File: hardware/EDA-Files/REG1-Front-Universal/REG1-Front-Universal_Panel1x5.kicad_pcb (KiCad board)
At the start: 2 copper layers, 106.3 x 52.8 mm, 60 parts, among them J1 Conn_02x04_Odd_Even, SW1 Prog, SW2 Func, SW3 Res, SW4 BL

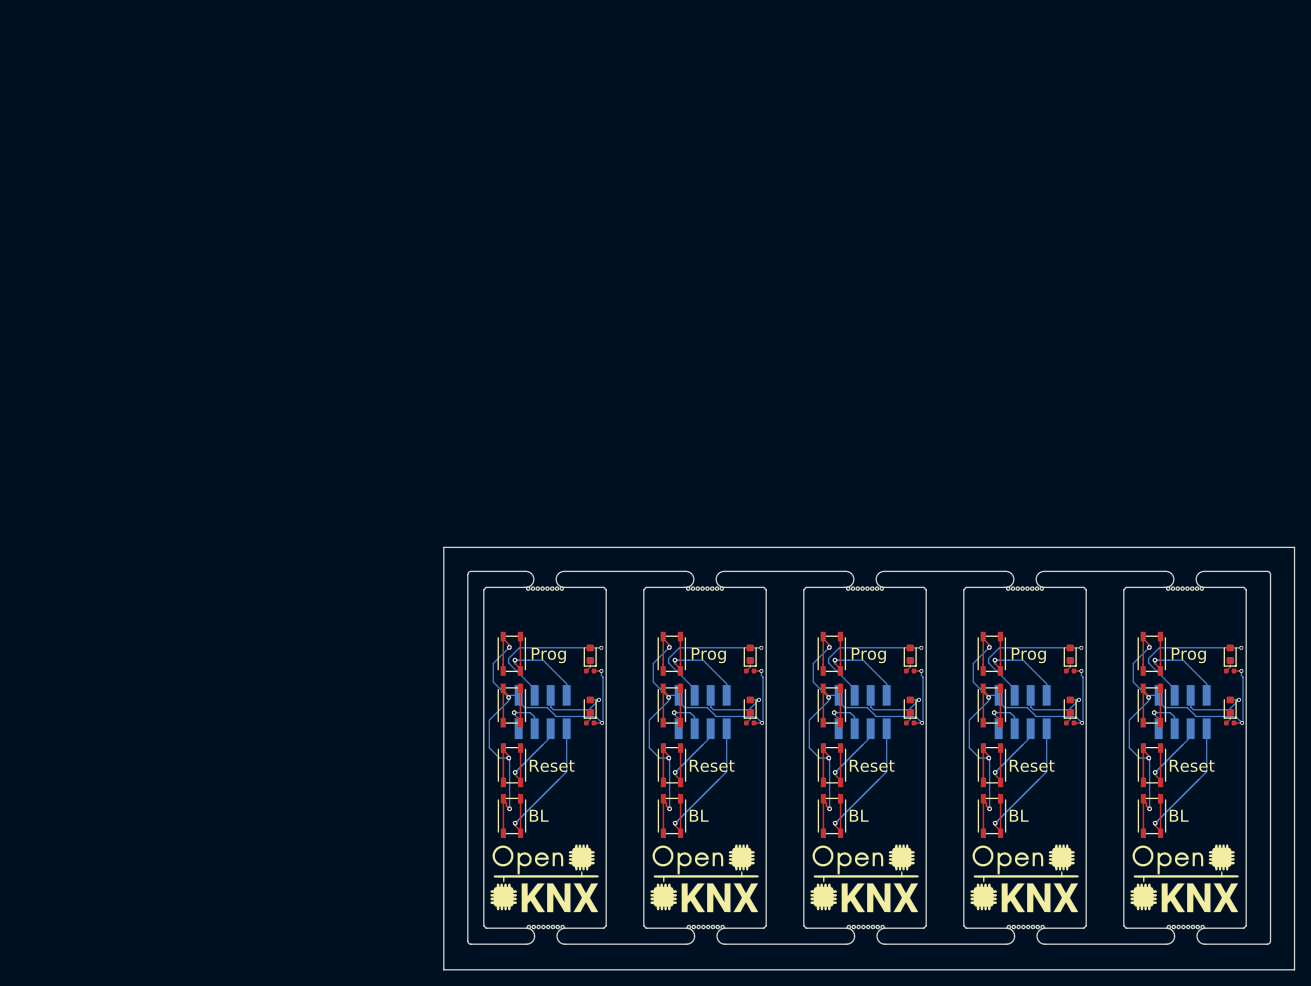
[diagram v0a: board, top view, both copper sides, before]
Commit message: REG1-Front-Universal V01.00
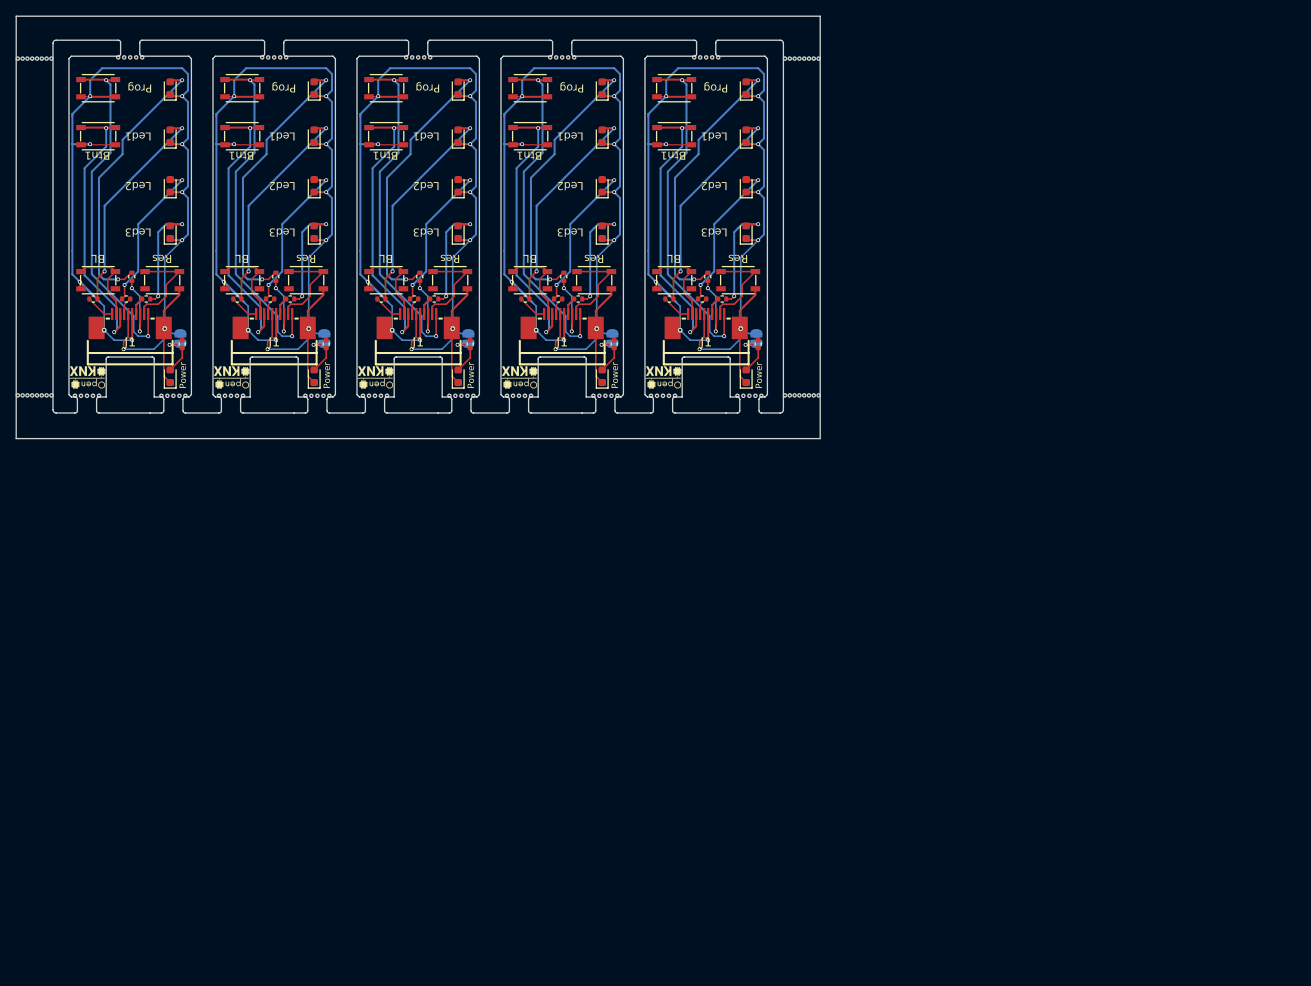
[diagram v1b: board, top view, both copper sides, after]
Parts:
- removed the D1 at (191.5, 117.8)
- removed the D1 at (171.5, 117.8)
- removed the D1 at (151.5, 117.8)
- removed the D1 at (131.5, 117.8)
- removed the D2 at (191.5, 124.2)
- removed the D2 at (171.5, 124.2)
- removed the D2 at (151.5, 124.2)
- removed the D2 at (131.5, 124.2)
- removed the G*** at (185.8, 146.4)
- removed the G*** at (165.8, 146.4)
- removed the G*** at (145.8, 146.4)
- removed the G*** at (125.8, 146.4)
- removed the G*** at (105.8, 146.4)
- removed the J1 at (185.6, 125.0)
- removed the J1 at (165.6, 125.0)
- removed the J1 at (145.6, 125.0)
- removed the J1 at (125.6, 125.0)
- removed the J1 at (105.6, 125.0)
- removed the R1 at (191.5, 119.8)
- removed the R1 at (171.5, 119.8)
- removed the R1 at (151.5, 119.8)
- removed the R1 at (131.5, 119.8)
- removed the R2 at (191.5, 126.3)
- removed the R2 at (171.5, 126.3)
- removed the R2 at (151.5, 126.3)
- removed the R2 at (131.5, 126.3)
- removed the SW1 at (181.7, 117.7)
- removed the SW1 at (161.7, 117.7)
- removed the SW1 at (141.7, 117.7)
- removed the SW1 at (121.7, 117.7)
- removed the SW2 at (181.7, 124.2)
- removed the SW2 at (161.7, 124.2)
- removed the SW2 at (141.7, 124.2)
- removed the SW2 at (121.7, 124.2)
- removed the SW3 at (181.7, 131.6)
- removed the SW3 at (161.7, 131.6)
- removed the SW3 at (141.7, 131.6)
- removed the SW3 at (121.7, 131.6)
- removed the SW4 at (181.7, 138.0)
- removed the SW4 at (161.7, 138.0)
- removed the SW4 at (141.7, 138.0)
- removed the SW4 at (121.7, 138.0)
- removed the mouse-bite at (186.4, 151.8)
- removed the mouse-bite at (105.3, 109.5)
- removed the mouse-bite at (166.4, 151.8)
- removed the mouse-bite at (146.4, 151.8)
- removed the mouse-bite at (126.5, 151.8)
- removed the mouse-bite at (185.3, 109.5)
- removed the mouse-bite at (165.3, 109.5)
- removed the mouse-bite at (145.3, 109.5)
- removed the mouse-bite at (125.3, 109.5)
- removed the mouse-bite at (106.5, 151.8)
- added D1: Prog, LED_SMD:LED_0603_1608Metric, F.Cu at (131.0, 47.0)
- added D1: Prog, LED_SMD:LED_0603_1608Metric, F.Cu at (77.0, 47.0)
- added D1: Prog, LED_SMD:LED_0603_1608Metric, F.Cu at (113.0, 47.0)
- added D1: Prog, LED_SMD:LED_0603_1608Metric, F.Cu at (95.0, 47.0)
- added D2: Led1, LED_SMD:LED_0603_1608Metric, F.Cu at (131.0, 53.0)
- added D2: Led1, LED_SMD:LED_0603_1608Metric, F.Cu at (95.0, 53.0)
- added D2: Led1, LED_SMD:LED_0603_1608Metric, F.Cu at (113.0, 53.0)
- added D2: Led1, LED_SMD:LED_0603_1608Metric, F.Cu at (77.0, 53.0)
- added D3: Led2, LED_SMD:LED_0603_1608Metric, F.Cu at (59.0, 59.2)
- added D3: Led2, LED_SMD:LED_0603_1608Metric, F.Cu at (95.0, 59.2)
- added D3: Led2, LED_SMD:LED_0603_1608Metric, F.Cu at (77.0, 59.2)
- added D3: Led2, LED_SMD:LED_0603_1608Metric, F.Cu at (113.0, 59.2)
- added D3: Led2, LED_SMD:LED_0603_1608Metric, F.Cu at (131.0, 59.2)
- added D4: Led3, LED_SMD:LED_0603_1608Metric, F.Cu at (131.0, 65.0)
- added D4: Led3, LED_SMD:LED_0603_1608Metric, F.Cu at (113.0, 65.0)
- added D4: Led3, LED_SMD:LED_0603_1608Metric, F.Cu at (95.0, 65.0)
- added D4: Led3, LED_SMD:LED_0603_1608Metric, F.Cu at (77.0, 65.0)
- added D4: Led3, LED_SMD:LED_0603_1608Metric, F.Cu at (59.0, 65.0)
- added D5: Power, LED_SMD:LED_0603_1608Metric, F.Cu at (113.0, 83.0)
- added D5: Power, LED_SMD:LED_0603_1608Metric, F.Cu at (59.0, 83.0)
- added D5: Power, LED_SMD:LED_0603_1608Metric, F.Cu at (95.0, 83.0)
- added D5: Power, LED_SMD:LED_0603_1608Metric, F.Cu at (77.0, 83.0)
- added D5: Power, LED_SMD:LED_0603_1608Metric, F.Cu at (131.0, 83.0)
- added G***: LOGO, OpenKNX:OpenKNX_Logo_05x03, F.Cu at (120.7, 83.0)
- added G***: LOGO, OpenKNX:OpenKNX_Logo_07x05, B.Cu at (106.0, 50.6)
- added G***: LOGO, OpenKNX:OpenKNX_Logo_05x03, F.Cu at (66.7, 83.0)
- added G***: LOGO, OpenKNX:OpenKNX_Logo_05x03, F.Cu at (102.7, 83.0)
- added G***: LOGO, OpenKNX:OpenKNX_Logo_05x03, F.Cu at (84.7, 83.0)
- added G***: LOGO, OpenKNX:OpenKNX_Logo_05x03, F.Cu at (48.7, 83.0)
- added G***: LOGO, OpenKNX:OpenKNX_Logo_07x05, B.Cu at (70.0, 50.6)
- added G***: LOGO, OpenKNX:OpenKNX_Logo_07x05, B.Cu at (88.0, 50.6)
- added G***: LOGO, OpenKNX:OpenKNX_Logo_07x05, B.Cu at (52.0, 50.6)
- added G***: LOGO, OpenKNX:OpenKNX_Logo_07x05, B.Cu at (124.0, 50.6)
- added J1: Frontpanel, EasyEDAModLib:C11050_FPC-SMD_P0.5-10P_LSXJ-H2.0-10P, F.Cu at (72.0, 76.1)
- added J1: Frontpanel, EasyEDAModLib:C11050_FPC-SMD_P0.5-10P_LSXJ-H2.0-10P, F.Cu at (54.0, 76.1)
- added J1: Frontpanel, EasyEDAModLib:C11050_FPC-SMD_P0.5-10P_LSXJ-H2.0-10P, F.Cu at (90.0, 76.1)
- added J1: Frontpanel, EasyEDAModLib:C11050_FPC-SMD_P0.5-10P_LSXJ-H2.0-10P, F.Cu at (108.0, 76.1)
- added J1: Frontpanel, EasyEDAModLib:C11050_FPC-SMD_P0.5-10P_LSXJ-H2.0-10P, F.Cu at (126.0, 76.1)
- added JP1: PowerLED Jumper, Jumper:SolderJumper-2_P1.3mm_Open_RoundedPad1.0x1.5mm, B.Cu at (60.3, 78.3)
- added JP1: PowerLED Jumper, Jumper:SolderJumper-2_P1.3mm_Open_RoundedPad1.0x1.5mm, B.Cu at (114.3, 78.3)
- added JP1: PowerLED Jumper, Jumper:SolderJumper-2_P1.3mm_Open_RoundedPad1.0x1.5mm, B.Cu at (96.3, 78.3)
- added JP1: PowerLED Jumper, Jumper:SolderJumper-2_P1.3mm_Open_RoundedPad1.0x1.5mm, B.Cu at (132.3, 78.3)
- added JP1: PowerLED Jumper, Jumper:SolderJumper-2_P1.3mm_Open_RoundedPad1.0x1.5mm, B.Cu at (78.3, 78.3)
- added R1: 2k2, Resistor_SMD:R_0402_1005Metric, F.Cu at (126.2, 70.6)
- added R1: 2k2, Resistor_SMD:R_0402_1005Metric, F.Cu at (72.2, 70.6)
- added R1: 2k2, Resistor_SMD:R_0402_1005Metric, F.Cu at (108.2, 70.6)
- added R1: 2k2, Resistor_SMD:R_0402_1005Metric, F.Cu at (90.2, 70.6)
- added R2: 2k2, Resistor_SMD:R_0402_1005Metric, F.Cu at (121.4, 73.3)
- added R2: 2k2, Resistor_SMD:R_0402_1005Metric, F.Cu at (85.4, 73.3)
- added R2: 2k2, Resistor_SMD:R_0402_1005Metric, F.Cu at (103.4, 73.3)
- added R2: 2k2, Resistor_SMD:R_0402_1005Metric, F.Cu at (67.4, 73.3)
- added R3: 2k2, Resistor_SMD:R_0402_1005Metric, F.Cu at (89.5, 73.3)
- added R3: 2k2, Resistor_SMD:R_0402_1005Metric, F.Cu at (107.5, 73.3)
- added R3: 2k2, Resistor_SMD:R_0402_1005Metric, F.Cu at (71.5, 73.3)
- added R3: 2k2, Resistor_SMD:R_0402_1005Metric, F.Cu at (53.5, 73.3)
- added R3: 2k2, Resistor_SMD:R_0402_1005Metric, F.Cu at (125.5, 73.3)
- added R4: 2k2, Resistor_SMD:R_0402_1005Metric, F.Cu at (56.0, 73.3)
- added R4: 2k2, Resistor_SMD:R_0402_1005Metric, F.Cu at (110.0, 73.3)
- added R4: 2k2, Resistor_SMD:R_0402_1005Metric, F.Cu at (92.0, 73.3)
- added R4: 2k2, Resistor_SMD:R_0402_1005Metric, F.Cu at (74.0, 73.3)
- added R4: 2k2, Resistor_SMD:R_0402_1005Metric, F.Cu at (128.0, 73.3)
- added R5: 2k2, Resistor_SMD:R_0402_1005Metric, F.Cu at (132.5, 79.0)
- added R5: 2k2, Resistor_SMD:R_0402_1005Metric, F.Cu at (114.5, 79.0)
- added R5: 2k2, Resistor_SMD:R_0402_1005Metric, F.Cu at (96.5, 79.0)
- added R5: 2k2, Resistor_SMD:R_0402_1005Metric, F.Cu at (60.5, 79.0)
- added R5: 2k2, Resistor_SMD:R_0402_1005Metric, F.Cu at (78.5, 79.0)
- added SW1: Prog, EasyEDAModLib:C455282_SW-SMD_4P-L4.2-W3.3-P2.15-LS5.1, F.Cu at (104.0, 47.0)
- added SW1: Prog, EasyEDAModLib:C455282_SW-SMD_4P-L4.2-W3.3-P2.15-LS5.1, F.Cu at (122.0, 47.0)
- added SW1: Prog, EasyEDAModLib:C455282_SW-SMD_4P-L4.2-W3.3-P2.15-LS5.1, F.Cu at (86.0, 47.0)
- added SW1: Prog, EasyEDAModLib:C455282_SW-SMD_4P-L4.2-W3.3-P2.15-LS5.1, F.Cu at (68.0, 47.0)
- added SW2: Btn1, EasyEDAModLib:C455282_SW-SMD_4P-L4.2-W3.3-P2.15-LS5.1, F.Cu at (86.0, 53.0)
- added SW2: Btn1, EasyEDAModLib:C455282_SW-SMD_4P-L4.2-W3.3-P2.15-LS5.1, F.Cu at (104.0, 53.0)
- added SW2: Btn1, EasyEDAModLib:C455282_SW-SMD_4P-L4.2-W3.3-P2.15-LS5.1, F.Cu at (122.0, 53.0)
- added SW2: Btn1, EasyEDAModLib:C455282_SW-SMD_4P-L4.2-W3.3-P2.15-LS5.1, F.Cu at (68.0, 53.0)
- added SW3: Res, EasyEDAModLib:C455282_SW-SMD_4P-L4.2-W3.3-P2.15-LS5.1, F.Cu at (76.0, 71.0)
- added SW3: Res, EasyEDAModLib:C455282_SW-SMD_4P-L4.2-W3.3-P2.15-LS5.1, F.Cu at (94.0, 71.0)
- added SW3: Res, EasyEDAModLib:C455282_SW-SMD_4P-L4.2-W3.3-P2.15-LS5.1, F.Cu at (130.0, 71.0)
- added SW3: Res, EasyEDAModLib:C455282_SW-SMD_4P-L4.2-W3.3-P2.15-LS5.1, F.Cu at (112.0, 71.0)
- added SW4: BL, EasyEDAModLib:C455282_SW-SMD_4P-L4.2-W3.3-P2.15-LS5.1, F.Cu at (68.0, 71.0)
- added SW4: BL, EasyEDAModLib:C455282_SW-SMD_4P-L4.2-W3.3-P2.15-LS5.1, F.Cu at (122.0, 71.0)
- added SW4: BL, EasyEDAModLib:C455282_SW-SMD_4P-L4.2-W3.3-P2.15-LS5.1, F.Cu at (104.0, 71.0)
- added SW4: BL, EasyEDAModLib:C455282_SW-SMD_4P-L4.2-W3.3-P2.15-LS5.1, F.Cu at (86.0, 71.0)
- added e: VAL**, DomsKiCADLib:mouse-bite-5.00mm-frame, F.Cu at (41.5, 43.3)
- added e: VAL**, DomsKiCADLib:mouse-bite-5.00mm-frame, F.Cu at (137.4, 43.3)
- added mouse-bite: mouse-bite-2.00mm-slot_1side, DomsKiCADLib:mouse-bite-2.00mm-slot_1side, F.Cu at (48.6, 86.2)
- added mouse-bite: mouse-bite-2.00mm-slot_1side, DomsKiCADLib:mouse-bite-2.00mm-slot_1side, F.Cu at (131.4, 86.2)
- added mouse-bite: VAL**, DomsKiCADLib:mouse-bite-5.00mm-frame, F.Cu at (137.4, 85.4)
- added mouse-bite: mouse-bite-2.00mm-slot_1side, DomsKiCADLib:mouse-bite-2.00mm-slot_1side, F.Cu at (54.0, 42.4)
- added mouse-bite: mouse-bite-2.00mm-slot_1side, DomsKiCADLib:mouse-bite-2.00mm-slot_1side, F.Cu at (95.4, 86.2)
- added mouse-bite: mouse-bite-2.00mm-slot_1side, DomsKiCADLib:mouse-bite-2.00mm-slot_1side, F.Cu at (72.0, 42.4)
- added mouse-bite: mouse-bite-2.00mm-slot_1side, DomsKiCADLib:mouse-bite-2.00mm-slot_1side, F.Cu at (66.6, 86.2)
- added mouse-bite: mouse-bite-2.00mm-slot_1side, DomsKiCADLib:mouse-bite-2.00mm-slot_1side, F.Cu at (126.0, 42.4)
- added mouse-bite: mouse-bite-2.00mm-slot_1side, DomsKiCADLib:mouse-bite-2.00mm-slot_1side, F.Cu at (84.6, 86.2)
- added mouse-bite: mouse-bite-2.00mm-slot_1side, DomsKiCADLib:mouse-bite-2.00mm-slot_1side, F.Cu at (77.4, 86.2)
- added mouse-bite: VAL**, DomsKiCADLib:mouse-bite-5.00mm-frame, F.Cu at (41.5, 85.4)
- added mouse-bite: mouse-bite-2.00mm-slot_1side, DomsKiCADLib:mouse-bite-2.00mm-slot_1side, F.Cu at (120.6, 86.2)
- added mouse-bite: mouse-bite-2.00mm-slot_1side, DomsKiCADLib:mouse-bite-2.00mm-slot_1side, F.Cu at (113.4, 86.2)
- added mouse-bite: mouse-bite-2.00mm-slot_1side, DomsKiCADLib:mouse-bite-2.00mm-slot_1side, F.Cu at (108.0, 42.4)
- added mouse-bite: mouse-bite-2.00mm-slot_1side, DomsKiCADLib:mouse-bite-2.00mm-slot_1side, F.Cu at (59.4, 86.2)
- added mouse-bite: mouse-bite-2.00mm-slot_1side, DomsKiCADLib:mouse-bite-2.00mm-slot_1side, F.Cu at (102.6, 86.2)
- added mouse-bite: mouse-bite-2.00mm-slot_1side, DomsKiCADLib:mouse-bite-2.00mm-slot_1side, F.Cu at (90.0, 42.4)
- D2: value Func -> Led1
- R1, R2: value R -> 2k2
- SW1, SW3, SW4: footprint sirsydom:SW_Push_Xunpu_TS-1089S -> EasyEDAModLib:C455282_SW-SMD_4P-L4.2-W3.3-P2.15-LS5.1
- SW2: value Func -> Btn1; footprint sirsydom:SW_Push_Xunpu_TS-1089S -> EasyEDAModLib:C455282_SW-SMD_4P-L4.2-W3.3-P2.15-LS5.1
- moved D2 88.5 mm to (59.0, 53.0)
- moved D1 88.1 mm to (59.0, 47.0)
- moved SW2 88.0 mm to (50.0, 53.0), turned to 0 degrees
- moved SW1 87.6 mm to (50.0, 47.0), turned to 0 degrees
- moved SW4 84.6 mm to (50.0, 71.0), turned to 0 degrees
- moved R2 81.6 mm to (49.4, 73.3)
- moved R1 75.6 mm to (54.2, 70.6), turned to -90 degrees
- moved SW3 74.7 mm to (58.0, 71.0), turned to 0 degrees
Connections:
- D1 pad 1: Net-(D1-Pad1) -> GND
- D1 pad 2: PROGLED -> Net-(D1-A)
- D2 pad 1: Net-(D2-Pad1) -> GND
- D2 pad 2: GPIO03 -> Net-(D2-A)
- R1 pad 1: GND -> Net-(D1-A)
- R1 pad 2: Net-(D1-Pad1) -> GPIO25
- R2 pad 1: GND -> Net-(D2-A)
- R2 pad 2: Net-(D2-Pad1) -> GPIO6
- SW1 pad 1: PROGBTN -> GPIO23
- SW2 pad 1: GPIO24 -> GPIO7
- SW4 pad 1: BOOTSEL_F -> BOOTSEL
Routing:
- net GND: track 352.6 -> 606.9 mm, vias 30 -> 50
- net GPIO23: track 0.00 -> 219.8 mm, vias 0 -> 10
- net GPIO7: track 0.00 -> 176.6 mm, vias 0 -> 10
- net Net-(D1-A): track 0.00 -> 174.6 mm, vias 0 -> 10
- net BOOTSEL_F: track 140.1 -> 0.00 mm, vias 5 -> 0
- net Net-(D2-A): track 0.00 -> 137.0 mm, vias 0 -> 10
- net PROGLED: track 97.5 -> 0.00 mm, vias 5 -> 0
- net Net-(D3-A): track 0.00 -> 97.5 mm, vias 0 -> 10
- net PROGBTN: track 75.4 -> 0.00 mm, vias 5 -> 0
- net Net-(D4-A): track 0.00 -> 70.7 mm, vias 0 -> 10
- net +3.3V: track 0.00 -> 62.7 mm, vias 0 -> 5
- net BOOTSEL: track 0.00 -> 54.4 mm
- net GPIO03: track 46.3 -> 0.00 mm, vias 5 -> 0
- net GPIO25: track 0.00 -> 46.1 mm, vias 0 -> 10
- net GPIO24: track 50.5 -> 11.0 mm, vias 5 -> 0
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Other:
- board size 106.3 x 52.8 mm -> 100.5 x 52.8 mm
- net class Default removed
- rule pad_to_mask_clearance: 0.051 -> 0.038
- board text added: "REG1-Front-Universal V01.00 (c) Ing-Dom, 2023"
- board text removed: "3V3"
- board text removed: "BL"
- board text removed: "GND"
- board text removed: "GP24"
- board text removed: "GP3"
- board text removed: "PBTN"
- board text removed: "PLED"
- board text removed: "Prog"
- board text removed: "REG1-Front-Universal V00.02 © Ing-Dom, 2022"
- board text removed: "RES"
- board text removed: "Reset"

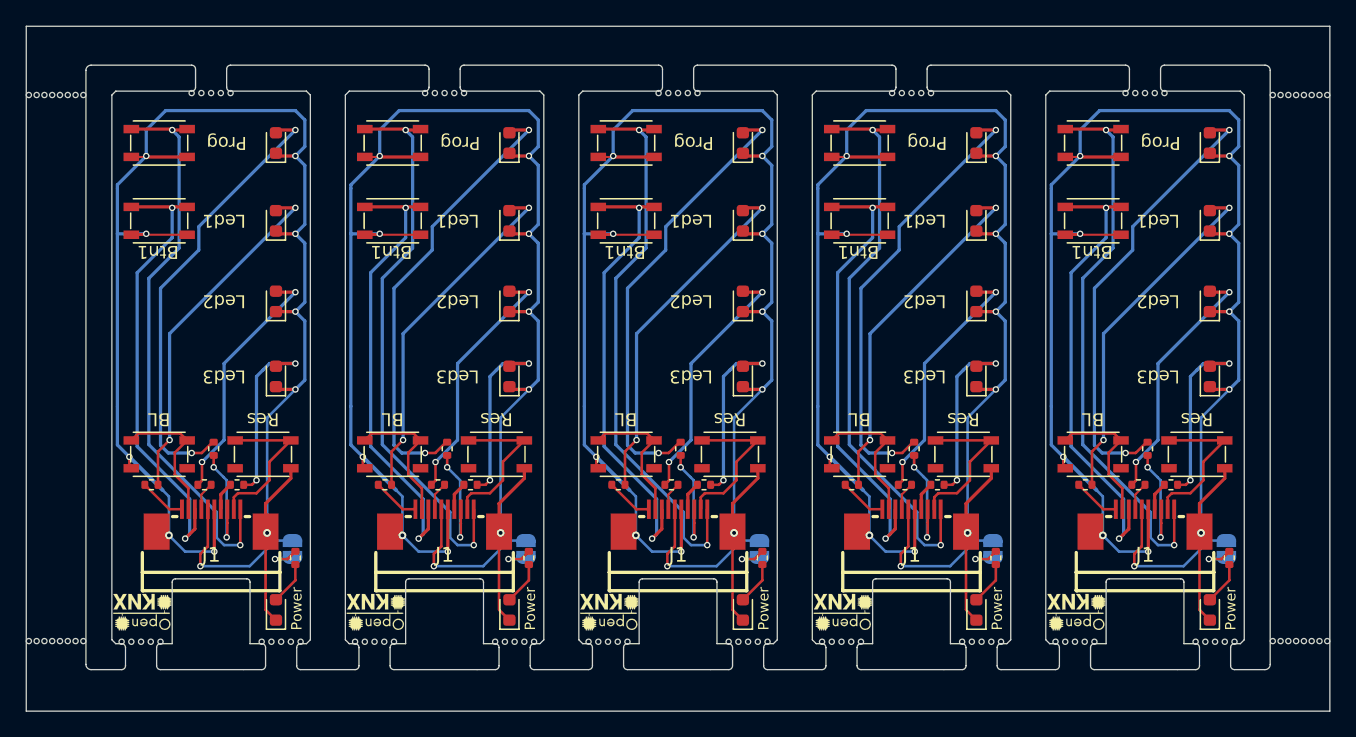
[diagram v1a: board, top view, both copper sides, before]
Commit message: new V01.00 (some 0.1 bigger)
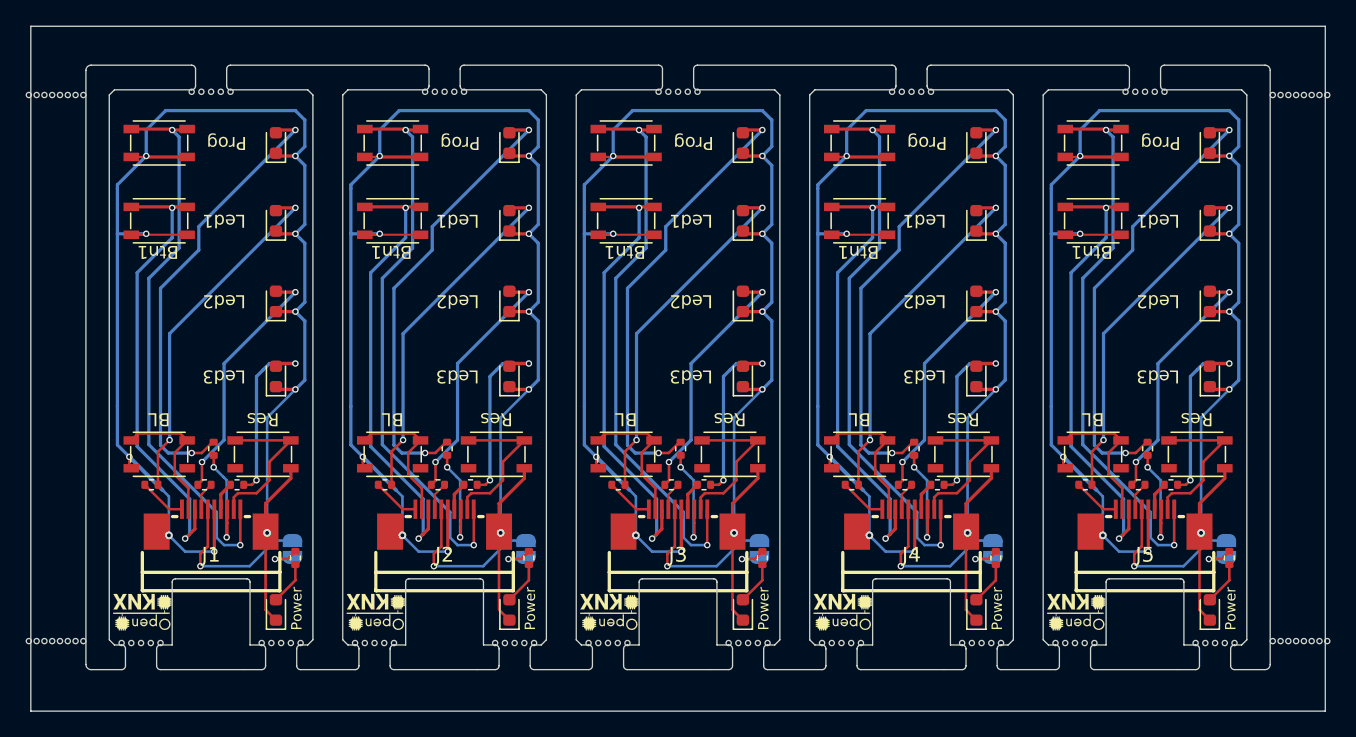
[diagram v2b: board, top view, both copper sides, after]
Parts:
- removed the D1 at (131.0, 47.0)
- removed the D1 at (77.0, 47.0)
- removed the D1 at (113.0, 47.0)
- removed the D1 at (95.0, 47.0)
- removed the D2 at (131.0, 53.0)
- removed the D2 at (95.0, 53.0)
- removed the D2 at (113.0, 53.0)
- removed the D2 at (77.0, 53.0)
- removed the D3 at (95.0, 59.2)
- removed the D3 at (77.0, 59.2)
- removed the D3 at (113.0, 59.2)
- removed the D3 at (131.0, 59.2)
- removed the D4 at (131.0, 65.0)
- removed the D4 at (113.0, 65.0)
- removed the D4 at (95.0, 65.0)
- removed the D4 at (77.0, 65.0)
- removed the D5 at (113.0, 83.0)
- removed the D5 at (95.0, 83.0)
- removed the D5 at (77.0, 83.0)
- removed the D5 at (131.0, 83.0)
- removed the G*** at (120.7, 83.0)
- removed the G*** at (106.0, 50.6)
- removed the G*** at (66.7, 83.0)
- removed the G*** at (102.7, 83.0)
- removed the G*** at (84.7, 83.0)
- removed the G*** at (70.0, 50.6)
- removed the G*** at (88.0, 50.6)
- removed the G*** at (124.0, 50.6)
- removed the J1 at (72.0, 76.1)
- removed the J1 at (90.0, 76.1)
- removed the J1 at (108.0, 76.1)
- removed the J1 at (126.0, 76.1)
- removed the JP1 at (114.3, 78.3)
- removed the JP1 at (96.3, 78.3)
- removed the JP1 at (132.3, 78.3)
- removed the JP1 at (78.3, 78.3)
- removed the R1 at (126.2, 70.6)
- removed the R1 at (72.2, 70.6)
- removed the R1 at (108.2, 70.6)
- removed the R1 at (90.2, 70.6)
- removed the R2 at (121.4, 73.3)
- removed the R2 at (85.4, 73.3)
- removed the R2 at (103.4, 73.3)
- removed the R2 at (67.4, 73.3)
- removed the R3 at (89.5, 73.3)
- removed the R3 at (107.5, 73.3)
- removed the R3 at (71.5, 73.3)
- removed the R3 at (125.5, 73.3)
- removed the R4 at (110.0, 73.3)
- removed the R4 at (92.0, 73.3)
- removed the R4 at (74.0, 73.3)
- removed the R4 at (128.0, 73.3)
- removed the R5 at (132.5, 79.0)
- removed the R5 at (114.5, 79.0)
- removed the R5 at (96.5, 79.0)
- removed the R5 at (78.5, 79.0)
- removed the SW1 at (104.0, 47.0)
- removed the SW1 at (122.0, 47.0)
- removed the SW1 at (86.0, 47.0)
- removed the SW1 at (68.0, 47.0)
- removed the SW2 at (86.0, 53.0)
- removed the SW2 at (104.0, 53.0)
- removed the SW2 at (122.0, 53.0)
- removed the SW2 at (68.0, 53.0)
- removed the SW3 at (76.0, 71.0)
- removed the SW3 at (94.0, 71.0)
- removed the SW3 at (130.0, 71.0)
- removed the SW3 at (112.0, 71.0)
- removed the SW4 at (68.0, 71.0)
- removed the SW4 at (122.0, 71.0)
- removed the SW4 at (104.0, 71.0)
- removed the SW4 at (86.0, 71.0)
- removed the mouse-bite at (131.4, 86.2)
- removed the mouse-bite at (95.4, 86.2)
- removed the mouse-bite at (72.0, 42.4)
- removed the mouse-bite at (66.6, 86.2)
- removed the mouse-bite at (126.0, 42.4)
- removed the mouse-bite at (84.6, 86.2)
- removed the mouse-bite at (77.4, 86.2)
- removed the mouse-bite at (120.6, 86.2)
- removed the mouse-bite at (113.4, 86.2)
- removed the mouse-bite at (108.0, 42.4)
- removed the mouse-bite at (102.6, 86.2)
- removed the mouse-bite at (90.0, 42.4)
- added D10: Power, LED_SMD:LED_0603_1608Metric, F.Cu at (77.0, 83.0)
- added D11: Prog, LED_SMD:LED_0603_1608Metric, F.Cu at (95.0, 47.0)
- added D12: Led1, LED_SMD:LED_0603_1608Metric, F.Cu at (95.0, 53.0)
- added D13: Led2, LED_SMD:LED_0603_1608Metric, F.Cu at (95.0, 59.2)
- added D14: Led3, LED_SMD:LED_0603_1608Metric, F.Cu at (95.0, 65.0)
- added D15: Power, LED_SMD:LED_0603_1608Metric, F.Cu at (95.0, 83.0)
- added D16: Prog, LED_SMD:LED_0603_1608Metric, F.Cu at (113.0, 47.0)
- added D17: Led1, LED_SMD:LED_0603_1608Metric, F.Cu at (113.0, 53.0)
- added D18: Led2, LED_SMD:LED_0603_1608Metric, F.Cu at (113.0, 59.2)
- added D19: Led3, LED_SMD:LED_0603_1608Metric, F.Cu at (113.0, 65.0)
- added D20: Power, LED_SMD:LED_0603_1608Metric, F.Cu at (113.0, 83.0)
- added D21: Prog, LED_SMD:LED_0603_1608Metric, F.Cu at (131.0, 47.0)
- added D22: Led1, LED_SMD:LED_0603_1608Metric, F.Cu at (131.0, 53.0)
- added D23: Led2, LED_SMD:LED_0603_1608Metric, F.Cu at (131.0, 59.2)
- added D24: Led3, LED_SMD:LED_0603_1608Metric, F.Cu at (131.0, 65.0)
- added D25: Power, LED_SMD:LED_0603_1608Metric, F.Cu at (131.0, 83.0)
- added D6: Prog, LED_SMD:LED_0603_1608Metric, F.Cu at (77.0, 47.0)
- added D7: Led1, LED_SMD:LED_0603_1608Metric, F.Cu at (77.0, 53.0)
- added D8: Led2, LED_SMD:LED_0603_1608Metric, F.Cu at (77.0, 59.2)
- added D9: Led3, LED_SMD:LED_0603_1608Metric, F.Cu at (77.0, 65.0)
- added G***1: LOGO, OpenKNX:OpenKNX_Logo_05x03, F.Cu at (66.7, 83.0)
- added G***2: LOGO, OpenKNX:OpenKNX_Logo_07x05, B.Cu at (70.0, 50.6)
- added G***3: LOGO, OpenKNX:OpenKNX_Logo_05x03, F.Cu at (84.7, 83.0)
- added G***4: LOGO, OpenKNX:OpenKNX_Logo_07x05, B.Cu at (88.0, 50.6)
- added G***5: LOGO, OpenKNX:OpenKNX_Logo_05x03, F.Cu at (102.7, 83.0)
- added G***6: LOGO, OpenKNX:OpenKNX_Logo_07x05, B.Cu at (106.0, 50.6)
- added G***7: LOGO, OpenKNX:OpenKNX_Logo_05x03, F.Cu at (120.7, 83.0)
- added G***8: LOGO, OpenKNX:OpenKNX_Logo_07x05, B.Cu at (124.0, 50.6)
- added J2: Frontpanel, EasyEDAModLib:C11050_FPC-SMD_P0.5-10P_LSXJ-H2.0-10P, F.Cu at (72.0, 76.1)
- added J3: Frontpanel, EasyEDAModLib:C11050_FPC-SMD_P0.5-10P_LSXJ-H2.0-10P, F.Cu at (90.0, 76.1)
- added J4: Frontpanel, EasyEDAModLib:C11050_FPC-SMD_P0.5-10P_LSXJ-H2.0-10P, F.Cu at (108.0, 76.1)
- added J5: Frontpanel, EasyEDAModLib:C11050_FPC-SMD_P0.5-10P_LSXJ-H2.0-10P, F.Cu at (126.0, 76.1)
- added JP2: PowerLED Jumper, Jumper:SolderJumper-2_P1.3mm_Open_RoundedPad1.0x1.5mm, B.Cu at (78.3, 78.3)
- added JP3: PowerLED Jumper, Jumper:SolderJumper-2_P1.3mm_Open_RoundedPad1.0x1.5mm, B.Cu at (96.3, 78.3)
- added JP4: PowerLED Jumper, Jumper:SolderJumper-2_P1.3mm_Open_RoundedPad1.0x1.5mm, B.Cu at (114.3, 78.3)
- added JP5: PowerLED Jumper, Jumper:SolderJumper-2_P1.3mm_Open_RoundedPad1.0x1.5mm, B.Cu at (132.3, 78.3)
- added R10: 2k2, Resistor_SMD:R_0402_1005Metric, F.Cu at (78.5, 79.0)
- added R11: 2k2, Resistor_SMD:R_0402_1005Metric, F.Cu at (90.2, 70.6)
- added R12: 2k2, Resistor_SMD:R_0402_1005Metric, F.Cu at (85.4, 73.3)
- added R13: 2k2, Resistor_SMD:R_0402_1005Metric, F.Cu at (89.5, 73.3)
- added R14: 2k2, Resistor_SMD:R_0402_1005Metric, F.Cu at (92.0, 73.3)
- added R15: 2k2, Resistor_SMD:R_0402_1005Metric, F.Cu at (96.5, 79.0)
- added R16: 2k2, Resistor_SMD:R_0402_1005Metric, F.Cu at (108.2, 70.6)
- added R17: 2k2, Resistor_SMD:R_0402_1005Metric, F.Cu at (103.4, 73.3)
- added R18: 2k2, Resistor_SMD:R_0402_1005Metric, F.Cu at (107.5, 73.3)
- added R19: 2k2, Resistor_SMD:R_0402_1005Metric, F.Cu at (110.0, 73.3)
- added R20: 2k2, Resistor_SMD:R_0402_1005Metric, F.Cu at (114.5, 79.0)
- added R21: 2k2, Resistor_SMD:R_0402_1005Metric, F.Cu at (126.2, 70.6)
- added R22: 2k2, Resistor_SMD:R_0402_1005Metric, F.Cu at (121.4, 73.3)
- added R23: 2k2, Resistor_SMD:R_0402_1005Metric, F.Cu at (125.5, 73.3)
- added R24: 2k2, Resistor_SMD:R_0402_1005Metric, F.Cu at (128.0, 73.3)
- added R25: 2k2, Resistor_SMD:R_0402_1005Metric, F.Cu at (132.5, 79.0)
- added R6: 2k2, Resistor_SMD:R_0402_1005Metric, F.Cu at (72.2, 70.6)
- added R7: 2k2, Resistor_SMD:R_0402_1005Metric, F.Cu at (67.4, 73.3)
- added R8: 2k2, Resistor_SMD:R_0402_1005Metric, F.Cu at (71.5, 73.3)
- added R9: 2k2, Resistor_SMD:R_0402_1005Metric, F.Cu at (74.0, 73.3)
- added SW10: Btn1, EasyEDAModLib:C455282_SW-SMD_4P-L4.2-W3.3-P2.15-LS5.1, F.Cu at (86.0, 53.0)
- added SW11: Res, EasyEDAModLib:C455282_SW-SMD_4P-L4.2-W3.3-P2.15-LS5.1, F.Cu at (94.0, 71.0)
- added SW12: BL, EasyEDAModLib:C455282_SW-SMD_4P-L4.2-W3.3-P2.15-LS5.1, F.Cu at (86.0, 71.0)
- added SW13: Prog, EasyEDAModLib:C455282_SW-SMD_4P-L4.2-W3.3-P2.15-LS5.1, F.Cu at (104.0, 47.0)
- added SW14: Btn1, EasyEDAModLib:C455282_SW-SMD_4P-L4.2-W3.3-P2.15-LS5.1, F.Cu at (104.0, 53.0)
- added SW15: Res, EasyEDAModLib:C455282_SW-SMD_4P-L4.2-W3.3-P2.15-LS5.1, F.Cu at (112.0, 71.0)
- added SW16: BL, EasyEDAModLib:C455282_SW-SMD_4P-L4.2-W3.3-P2.15-LS5.1, F.Cu at (104.0, 71.0)
- added SW17: Prog, EasyEDAModLib:C455282_SW-SMD_4P-L4.2-W3.3-P2.15-LS5.1, F.Cu at (122.0, 47.0)
- added SW18: Btn1, EasyEDAModLib:C455282_SW-SMD_4P-L4.2-W3.3-P2.15-LS5.1, F.Cu at (122.0, 53.0)
- added SW19: Res, EasyEDAModLib:C455282_SW-SMD_4P-L4.2-W3.3-P2.15-LS5.1, F.Cu at (130.0, 71.0)
- added SW20: BL, EasyEDAModLib:C455282_SW-SMD_4P-L4.2-W3.3-P2.15-LS5.1, F.Cu at (122.0, 71.0)
- added SW5: Prog, EasyEDAModLib:C455282_SW-SMD_4P-L4.2-W3.3-P2.15-LS5.1, F.Cu at (68.0, 47.0)
- added SW6: Btn1, EasyEDAModLib:C455282_SW-SMD_4P-L4.2-W3.3-P2.15-LS5.1, F.Cu at (68.0, 53.0)
- added SW7: Res, EasyEDAModLib:C455282_SW-SMD_4P-L4.2-W3.3-P2.15-LS5.1, F.Cu at (76.0, 71.0)
- added SW8: BL, EasyEDAModLib:C455282_SW-SMD_4P-L4.2-W3.3-P2.15-LS5.1, F.Cu at (68.0, 71.0)
- added SW9: Prog, EasyEDAModLib:C455282_SW-SMD_4P-L4.2-W3.3-P2.15-LS5.1, F.Cu at (86.0, 47.0)
- added mouse-bite1: mouse-bite-2.00mm-slot_1side, DomsKiCADLib:mouse-bite-2.00mm-slot_1side, F.Cu at (66.6, 86.3)
- added mouse-bite10: mouse-bite-2.00mm-slot_1side, DomsKiCADLib:mouse-bite-2.00mm-slot_1side, F.Cu at (120.6, 86.3)
- added mouse-bite11: mouse-bite-2.00mm-slot_1side, DomsKiCADLib:mouse-bite-2.00mm-slot_1side, F.Cu at (131.4, 86.3)
- added mouse-bite12: mouse-bite-2.00mm-slot_1side, DomsKiCADLib:mouse-bite-2.00mm-slot_1side, F.Cu at (126.0, 42.3)
- added mouse-bite2: mouse-bite-2.00mm-slot_1side, DomsKiCADLib:mouse-bite-2.00mm-slot_1side, F.Cu at (77.4, 86.3)
- added mouse-bite3: mouse-bite-2.00mm-slot_1side, DomsKiCADLib:mouse-bite-2.00mm-slot_1side, F.Cu at (72.0, 42.3)
- added mouse-bite4: mouse-bite-2.00mm-slot_1side, DomsKiCADLib:mouse-bite-2.00mm-slot_1side, F.Cu at (84.6, 86.3)
- added mouse-bite5: mouse-bite-2.00mm-slot_1side, DomsKiCADLib:mouse-bite-2.00mm-slot_1side, F.Cu at (95.4, 86.3)
- added mouse-bite6: mouse-bite-2.00mm-slot_1side, DomsKiCADLib:mouse-bite-2.00mm-slot_1side, F.Cu at (90.0, 42.3)
- added mouse-bite7: mouse-bite-2.00mm-slot_1side, DomsKiCADLib:mouse-bite-2.00mm-slot_1side, F.Cu at (102.6, 86.3)
- added mouse-bite8: mouse-bite-2.00mm-slot_1side, DomsKiCADLib:mouse-bite-2.00mm-slot_1side, F.Cu at (113.4, 86.3)
- added mouse-bite9: mouse-bite-2.00mm-slot_1side, DomsKiCADLib:mouse-bite-2.00mm-slot_1side, F.Cu at (108.0, 42.3)
- moved mouse-bite 0.10 mm to (54.0, 42.3)
- moved mouse-bite 0.10 mm to (48.6, 86.3)
- moved mouse-bite 0.10 mm to (59.4, 86.3)
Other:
- board size 100.5 x 52.8 mm -> 99.8 x 52.8 mm
